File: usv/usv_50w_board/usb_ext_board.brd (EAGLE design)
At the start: 10 x 13.6 mm, 3 parts

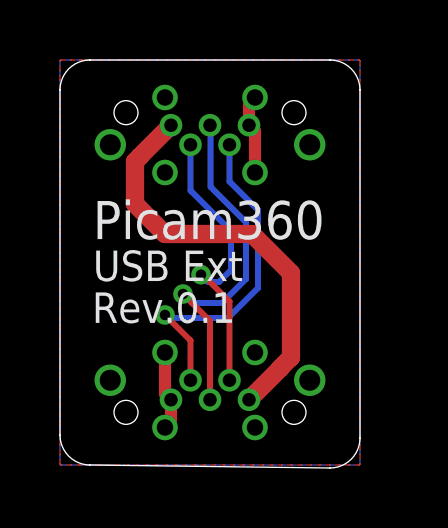
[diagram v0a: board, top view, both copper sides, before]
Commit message: usv50w
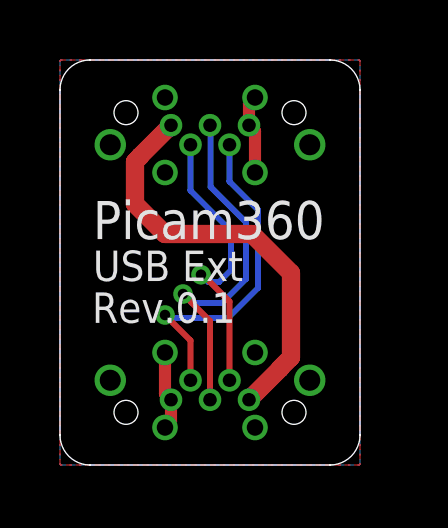
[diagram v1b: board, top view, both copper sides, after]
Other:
- board size 10 x 13.6 mm -> 10 x 13.5 mm
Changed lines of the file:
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@@
 <text x="1.099" y="6.132" size="1.016" layer="21">USB Ext</text>
 <text x="1.068" y="4.737" size="1.016" layer="21">Rev.0.1</text>
-<wire x1="1" y1="0" x2="9" y2="-0.1" width="0" layer="20"/>
-<wire x1="9" y1="-0.1" x2="10" y2="0.9" width="0" layer="20" curve="90"/>
-<wire x1="10" y1="0.9" x2="10" y2="12.5" width="0" layer="20"/>
+<wire x1="1" y1="0" x2="9" y2="0" width="0" layer="20"/>
+<wire x1="9" y1="0" x2="10" y2="1" width="0" layer="20" curve="90"/>
+<wire x1="10" y1="1" x2="10" y2="12.5" width="0" layer="20"/>
 <wire x1="10" y1="12.5" x2="9" y2="13.5" width="0" layer="20" curve="90"/>
 <wire x1="9" y1="13.5" x2="1" y2="13.5" width="0" layer="20"/>
